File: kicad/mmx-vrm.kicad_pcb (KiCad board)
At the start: 2 copper layers, 58.4 x 53 mm, 32 parts, among them J1 Conn_02x15_Row_Letter_First, Q1 Q_NPN_BEC, Q2 Q_NMOS_GDS, Q3 Q_NMOS_GDS, SW1 SW_DIP_x04, U1 NCP1579

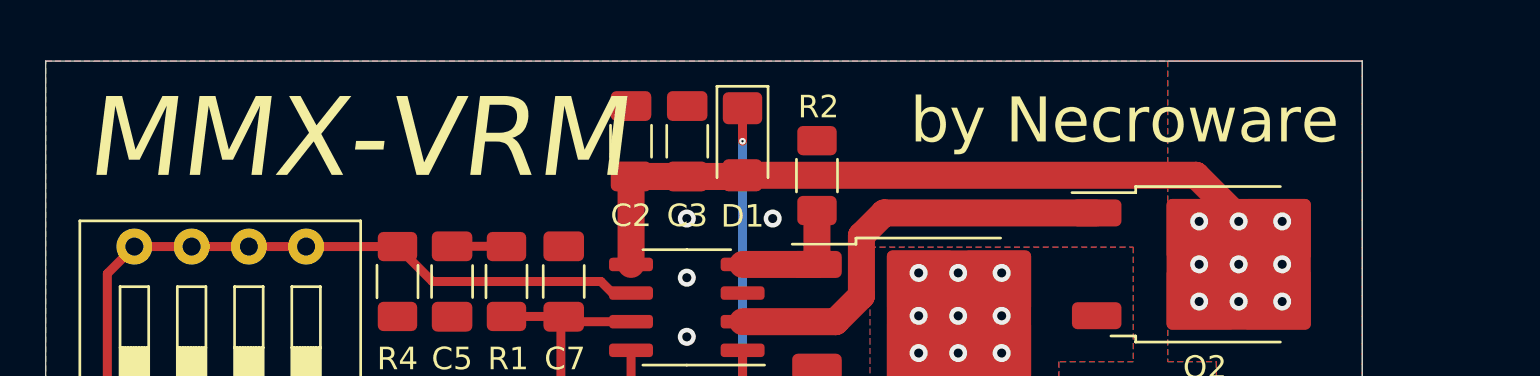
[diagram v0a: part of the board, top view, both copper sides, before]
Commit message: Updated parameters
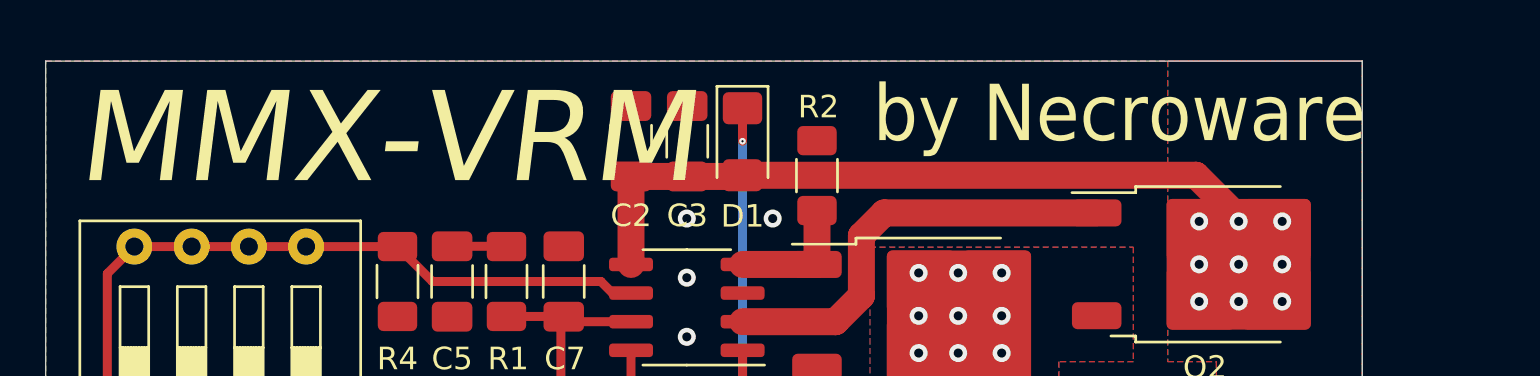
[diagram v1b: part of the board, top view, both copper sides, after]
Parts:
- R1: value 6,3K -> 15K
